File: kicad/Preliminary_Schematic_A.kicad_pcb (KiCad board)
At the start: 2 copper layers, 57.7 x 42 mm, 26 parts, among them J1 Battery Connection, J2 Load Cell System, M1 Motor_Servo, Q1 DMN2075U-7, U1 TOF

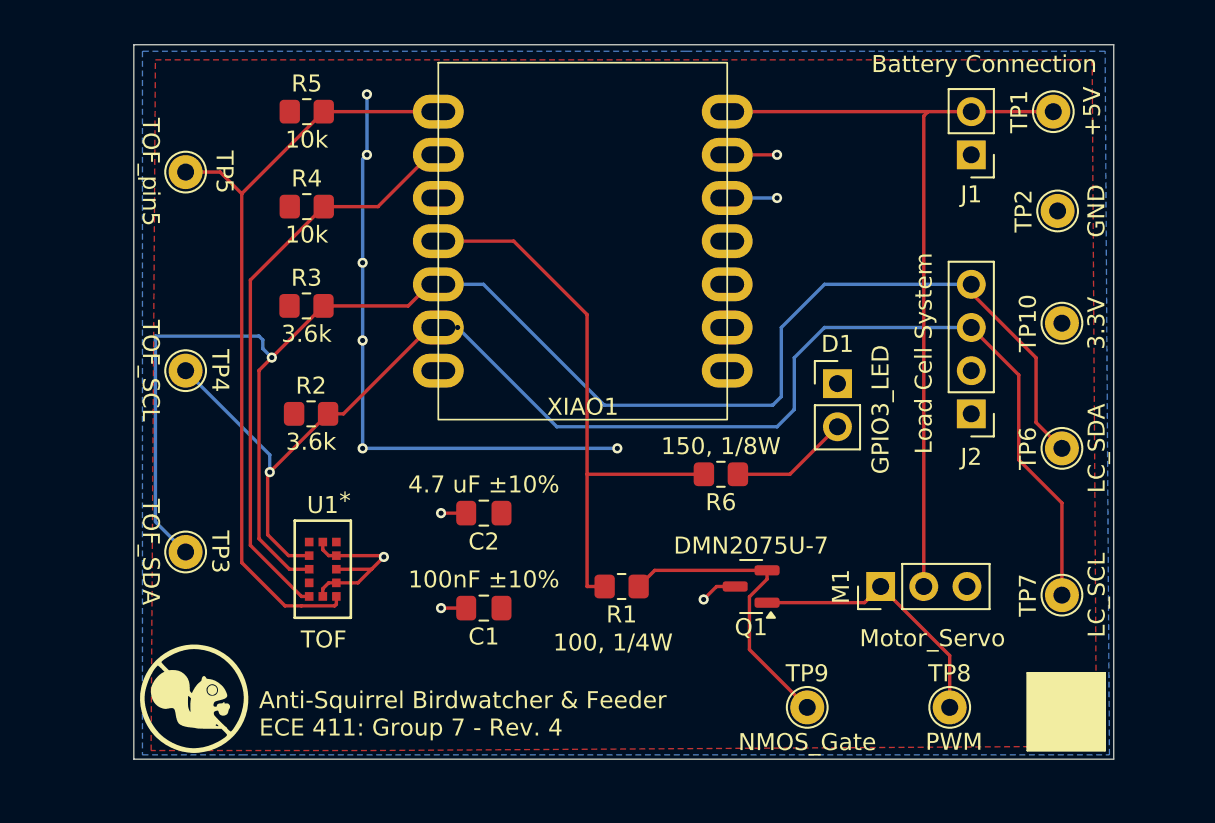
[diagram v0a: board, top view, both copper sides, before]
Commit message: Add files via upload
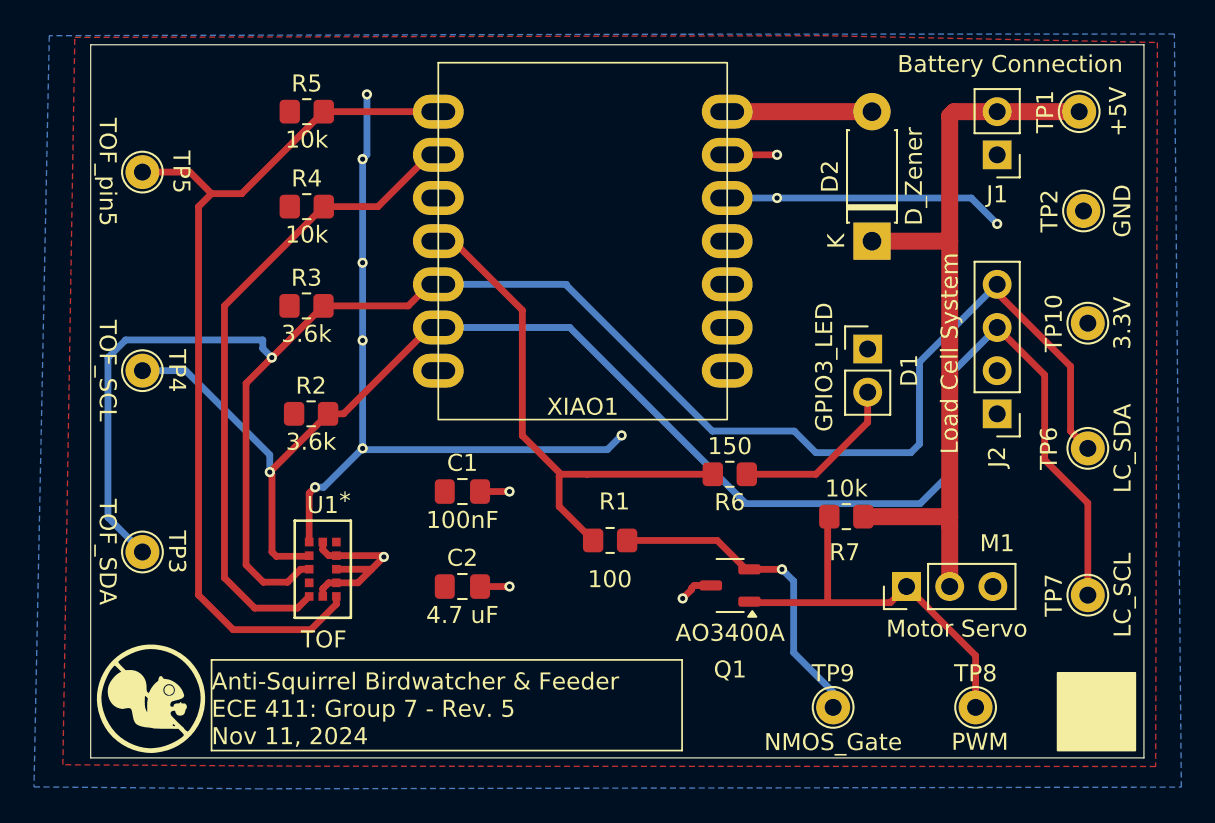
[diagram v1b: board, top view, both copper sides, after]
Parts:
- added D2: D_Zener, Diode_THT:D_DO-41_SOD81_P7.62mm_Horizontal, F.Cu at (165.6, 97.8)
- added R7: 10k, Resistor_SMD:R_0805_2012Metric_Pad1.20x1.40mm_HandSolder, F.Cu at (164.1, 114.0)
- C1: value 100nF ±10% -> 100nF
- C2: value 4.7 uF ±10% -> 4.7 uF
- M1: value Motor_Servo -> Motor Servo
- Q1: value DMN2075U-7 -> AO3400A; footprint Package_TO_SOT_SMD:SOT-23 -> Package_TO_SOT_SMD:SOT-23-3
- R1: value 100, 1/4W -> 100
- R6: value 150, 1/8W -> 150
- moved C1 6.97 mm to (141.5, 112.5), turned to 0 degrees
- moved C2 4.50 mm to (141.5, 118.1), turned to 0 degrees
- moved R1 2.79 mm to (150.2, 115.4)
- moved D1 2.70 mm to (165.4, 104.1)
- moved G*** 2.54 mm to (123.2, 124.7)
- moved TP3 2.54 mm to (122.7, 116.1)
- moved TP4 2.54 mm to (122.7, 105.4)
- moved TP5 2.54 mm to (122.7, 93.7)
- moved J1 1.52 mm to (173.0, 92.7)
- moved J2 1.52 mm to (173.0, 108.0)
- moved TP1 1.52 mm to (177.8, 90.2)
- moved TP10 1.52 mm to (178.3, 102.6)
- moved TP2 1.52 mm to (178.1, 96.0)
- moved TP6 1.52 mm to (178.3, 110.0)
- moved TP7 1.52 mm to (178.3, 118.6)
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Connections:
- XIAO1 pad 5V: +5V -> Net-(D2-A)
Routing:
- net /3.3V ESP32: track 38.8 -> 60.2 mm, vias 7 -> 9
- net Net-(J2-Pin_3): track 84.1 -> 95.0 mm, vias 2 -> 1
- net Net-(J2-Pin_4): track 100.0 -> 108.9 mm
- net Net-(D2-A): track 0.00 -> 8.52 mm
- net Net-(M1-PWM): track 15.9 -> 23.7 mm
- net Net-(U1-XSHUT): track 45.7 -> 53.4 mm
- net Net-(U1-GPIO1): track 33.9 -> 37.8 mm
- net Net-(R1-Pad2): track 35.0 -> 31.4 mm
- net Net-(D1-A): track 7.02 -> 10.2 mm
- net +5V: track 46.7 -> 45.1 mm
- net Net-(Q1-G): track 17.9 -> 19.0 mm, vias 0 -> 1
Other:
- board size 57.7 x 42 mm -> 62 x 42 mm
- board text added: "Anti-Squirrel Birdwatcher & Feeder ECE 411: Group 7 - Rev. 5 Nov 11, 2024"
- board text removed: "Anti-Squirrel Birdwatcher & Feeder ECE 411: Group 7 - Rev. 4"
